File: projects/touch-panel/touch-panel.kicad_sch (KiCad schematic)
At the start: 262 parts, among them J1 FPC-40P-0.5mm, Q1 AO3400, Q10 AO3400, Q100 AO3400, Q101 AO3400, Q102 AO3400, Q103 AO3400, Q104 AO3400, Q105 AO3400, Q106 AO3400, Q107 AO3400, Q108 AO3400, Q109 AO3400, Q11 AO3400, Q110 AO3400, Q111 AO3400, Q112 AO3400, Q113 AO3400, Q114 AO3400, Q115 AO3400, Q116 AO3400, Q117 AO3400, Q118 AO3400, Q119 AO3400, Q12 AO3400, Q120 AO3400, Q121 AO3400, Q122 AO3400, Q123 AO3400, Q124 AO3400, Q125 AO3400, Q126 AO3400, Q127 AO3400, Q128 AO3400, Q129 AO3400, Q13 AO3400, Q130 AO3400, Q131 AO3400, Q132 AO3400, Q133 AO3400, Q134 AO3400, Q135 AO3400, Q136 AO3400, Q137 AO3400, Q138 AO3400, Q139 AO3400, Q14 AO3400, Q140 AO3400, Q141 AO3400, Q142 AO3400, Q143 AO3400, Q144 AO3400, Q145 AO3400, Q146 AO3400, Q147 AO3400, Q148 AO3400, Q149 AO3400, Q15 AO3400, Q150 AO3400, Q151 AO3400, Q152 AO3400, Q153 AO3400, Q154 AO3400, Q155 AO3400, Q156 AO3400, Q157 AO3400, Q158 AO3400, Q159 AO3400, Q16 AO3400, Q160 AO3400, Q161 AO3400, Q162 AO3400, Q163 AO3400, Q164 AO3400, Q165 AO3400, Q166 AO3400, Q167 AO3400, Q168 AO3400, Q169 AO3400, Q17 AO3400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

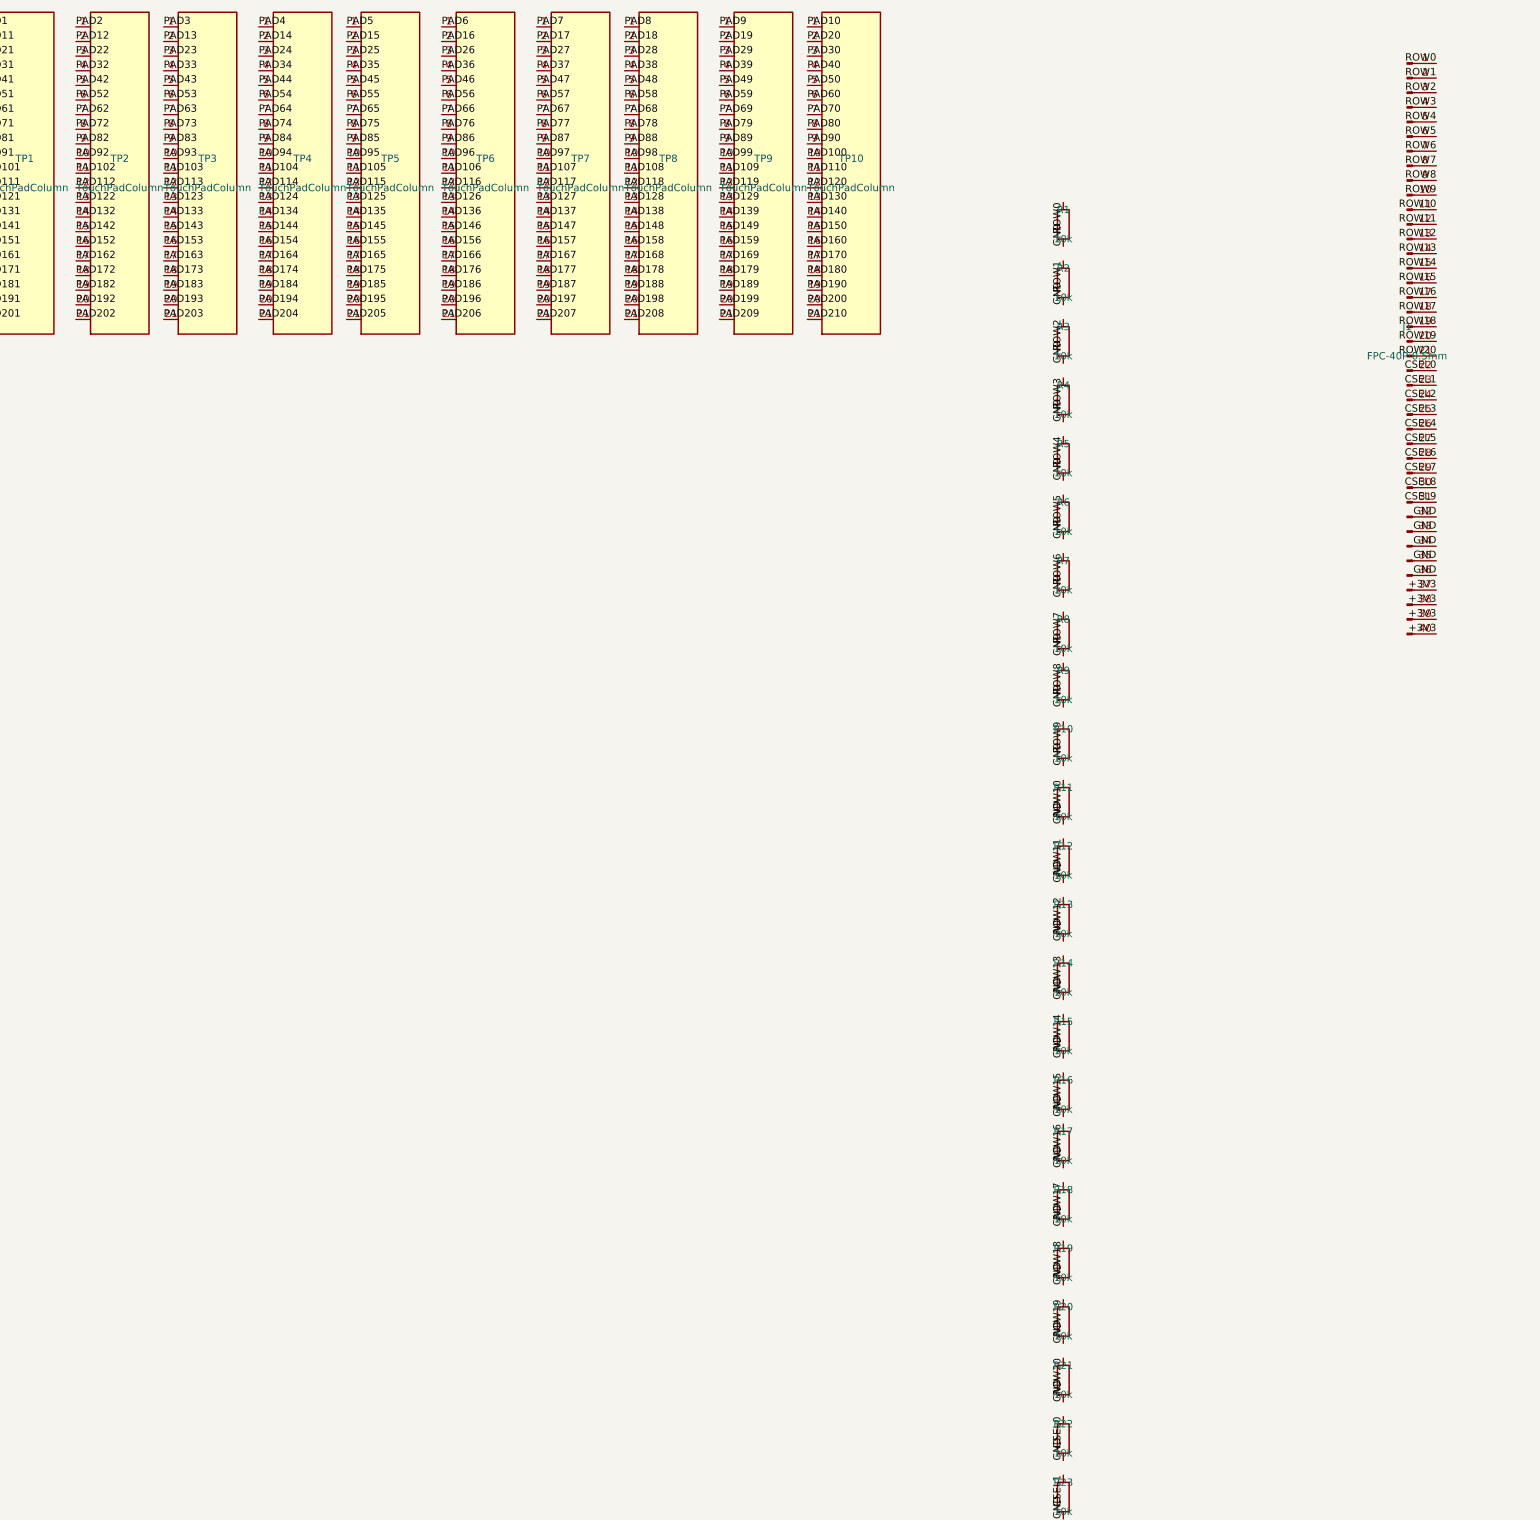
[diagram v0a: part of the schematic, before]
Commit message: 修改位置
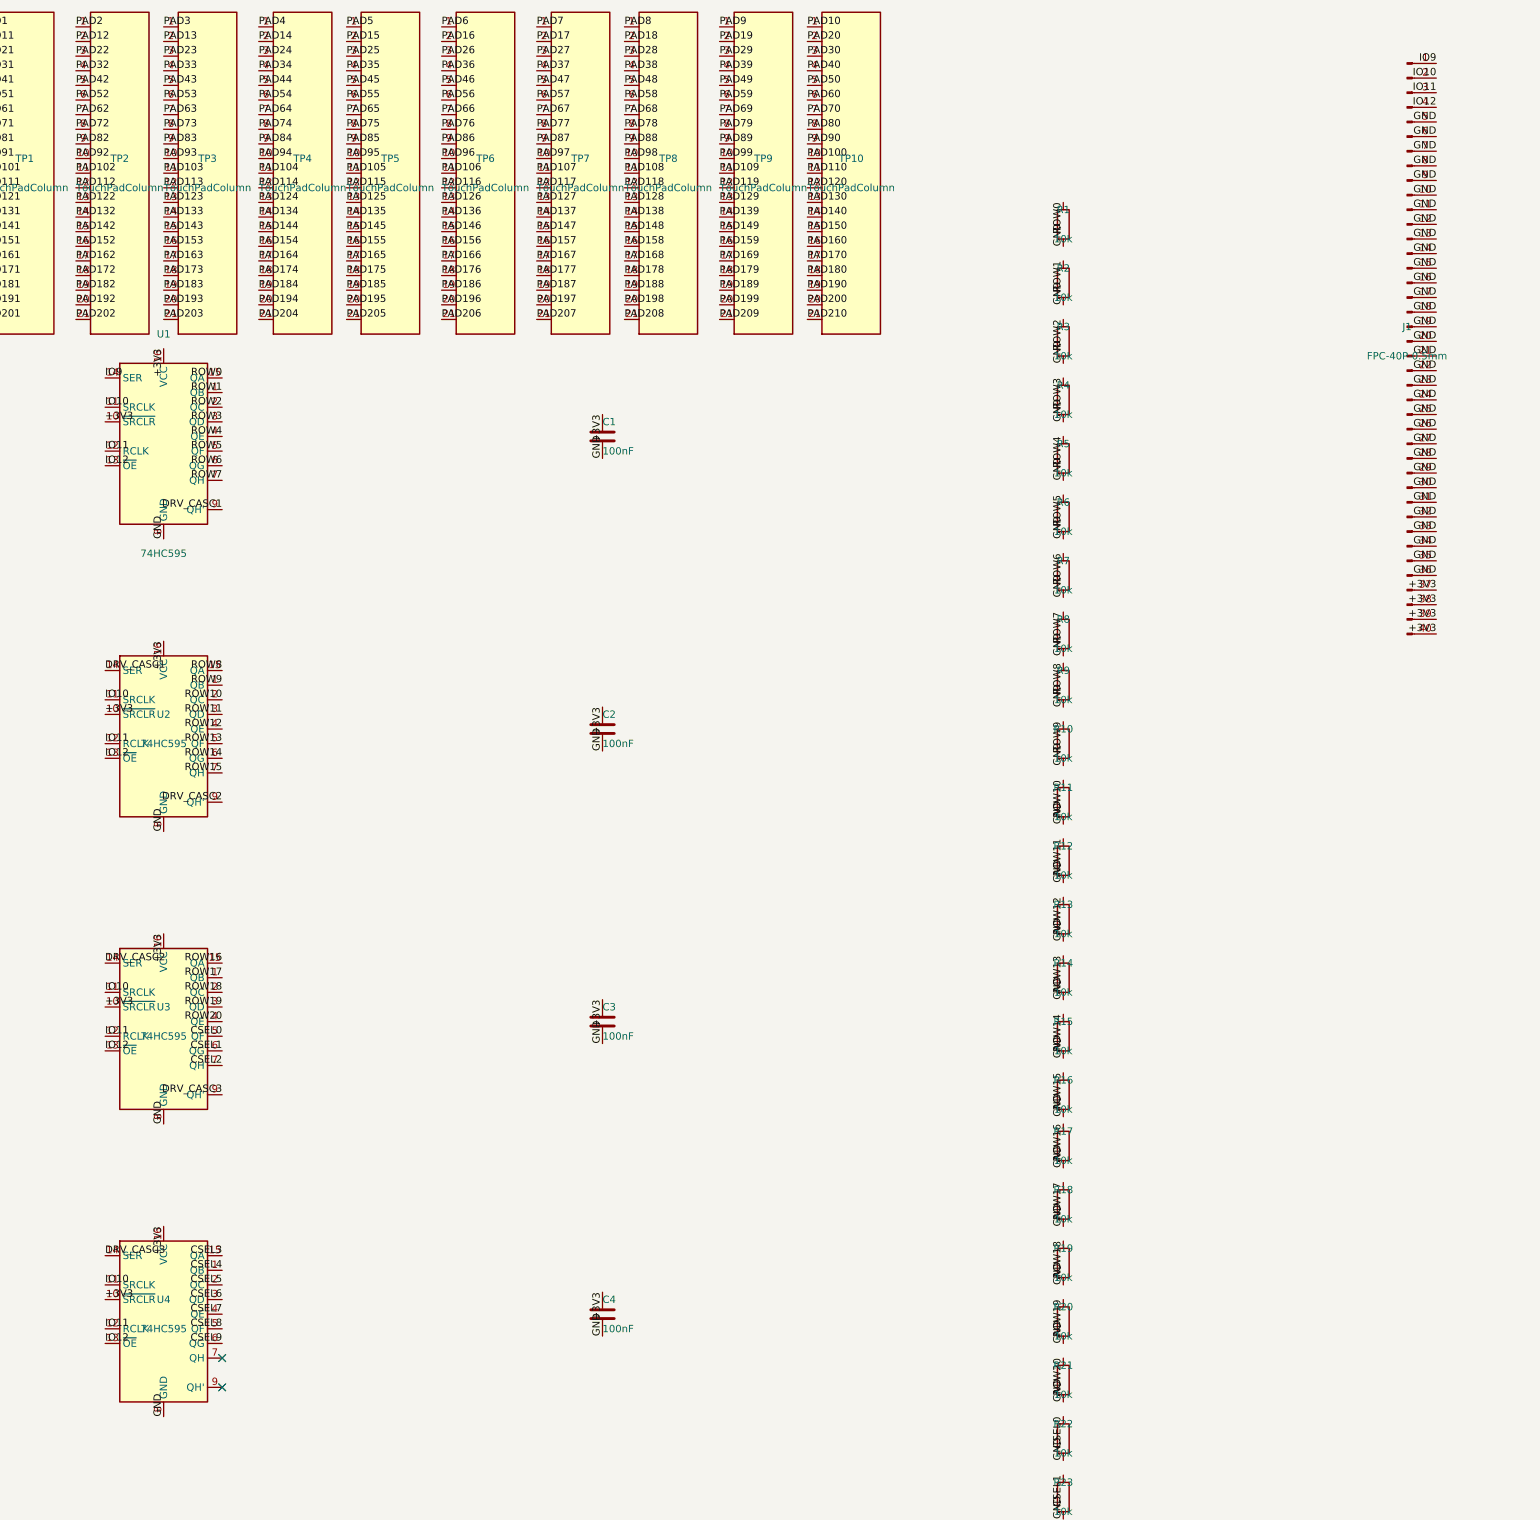
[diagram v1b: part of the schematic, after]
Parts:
- added C1, C2, C3, C4: 100nF, Capacitor_SMD:C_0402_1005Metric, symbol Device:C
- added U1, U2, U3, U4: 74HC595, Package_SO:SOIC-16_3.9x9.9mm_P1.27mm, symbol 74xx:74HC595
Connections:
- net +3V3: now also C1.1, C2.1, C3.1, C4.1, U1.10 (~{SRCLR}), U1.16 (VCC), U2.10 (~{SRCLR}), U2.16 (VCC), U3.10 (~{SRCLR}), U3.16 (VCC), U4.10 (~{SRCLR}), U4.16 (VCC)
- net CSEL0: now also U3.5 (QF); no longer J1.22 (Pin_22)
- net CSEL1: now also U3.6 (QG); no longer J1.23 (Pin_23)
- net CSEL2: now also U3.7 (QH); no longer J1.24 (Pin_24)
- net CSEL3: now also U4.15 (QA); no longer J1.25 (Pin_25)
- net CSEL4: now also U4.1 (QB); no longer J1.26 (Pin_26)
- net CSEL5: now also U4.2 (QC); no longer J1.27 (Pin_27)
- net CSEL6: now also U4.3 (QD); no longer J1.28 (Pin_28)
- net CSEL7: now also U4.4 (QE); no longer J1.29 (Pin_29)
- net CSEL8: now also U4.5 (QF); no longer J1.30 (Pin_30)
- net CSEL9: now also U4.6 (QG); no longer J1.31 (Pin_31)
- net GND: now also J1.10 (Pin_10), J1.11 (Pin_11), J1.12 (Pin_12), J1.13 (Pin_13), J1.14 (Pin_14), J1.15 (Pin_15), J1.16 (Pin_16), J1.17 (Pin_17), J1.18 (Pin_18), J1.19 (Pin_19), J1.20 (Pin_20), J1.21 (Pin_21), J1.22 (Pin_22), J1.23 (Pin_23), J1.24 (Pin_24), J1.25 (Pin_25), J1.26 (Pin_26), J1.27 (Pin_27), J1.28 (Pin_28), J1.29 (Pin_29), J1.30 (Pin_30), J1.31 (Pin_31), J1.5 (Pin_5), J1.6 (Pin_6), J1.7 (Pin_7), J1.8 (Pin_8), J1.9 (Pin_9), C1.2, C2.2, C3.2, C4.2, U1.8 (GND), U2.8 (GND), U3.8 (GND), U4.8 (GND)
- net ROW0: now also U1.15 (QA); no longer J1.1 (Pin_1)
- net ROW1: now also U1.1 (QB); no longer J1.2 (Pin_2)
- net ROW10: now also U2.2 (QC); no longer J1.11 (Pin_11)
- net ROW11: now also U2.3 (QD); no longer J1.12 (Pin_12)
- net ROW12: now also U2.4 (QE); no longer J1.13 (Pin_13)
- net ROW13: now also U2.5 (QF); no longer J1.14 (Pin_14)
- net ROW14: now also U2.6 (QG); no longer J1.15 (Pin_15)
- net ROW15: now also U2.7 (QH); no longer J1.16 (Pin_16)
- net ROW16: now also U3.15 (QA); no longer J1.17 (Pin_17)
- net ROW17: now also U3.1 (QB); no longer J1.18 (Pin_18)
- net ROW18: now also U3.2 (QC); no longer J1.19 (Pin_19)
- net ROW19: now also U3.3 (QD); no longer J1.20 (Pin_20)
- net ROW2: now also U1.2 (QC); no longer J1.3 (Pin_3)
- net ROW20: now also U3.4 (QE); no longer J1.21 (Pin_21)
- net ROW3: now also U1.3 (QD); no longer J1.4 (Pin_4)
- net ROW4: now also U1.4 (QE); no longer J1.5 (Pin_5)
- net ROW5: now also U1.5 (QF); no longer J1.6 (Pin_6)
- net ROW6: now also U1.6 (QG); no longer J1.7 (Pin_7)
- net ROW7: now also U1.7 (QH); no longer J1.8 (Pin_8)
- net ROW8: now also U2.15 (QA); no longer J1.9 (Pin_9)
- net ROW9: now also U2.1 (QB); no longer J1.10 (Pin_10)
- new net DRV_CASC1: U1.9 (QH'), U2.14 (SER)
- new net DRV_CASC2: U2.9 (QH'), U3.14 (SER)
- new net DRV_CASC3: U3.9 (QH'), U4.14 (SER)
- new net IO10: J1.2 (Pin_2), U1.11 (SRCLK), U2.11 (SRCLK), U3.11 (SRCLK), U4.11 (SRCLK)
- new net IO11: J1.3 (Pin_3), U1.12 (RCLK), U2.12 (RCLK), U3.12 (RCLK), U4.12 (RCLK)
- new net IO12: J1.4 (Pin_4), U1.13 (~{OE}), U2.13 (~{OE}), U3.13 (~{OE}), U4.13 (~{OE})
- new net IO9: J1.1 (Pin_1), U1.14 (SER)
- no-connect marks 0 -> 2
